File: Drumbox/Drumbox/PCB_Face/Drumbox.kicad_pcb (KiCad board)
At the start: 2 copper layers, 199.4 x 123.2 mm, 103 parts, among them J1 Bass IN, J10 HiHat IN, J12 Conn_01x08_Male, J15 Bass OUT, J16 HBonga OUT, J17 Snare OUT, J18 LBonga OUT, J19 Clave OUT, J2 HBonga IN, J20 HiHat OUT, J21 Conn_01x06_Male, J23 Conn_01x06_Male, J24 Conn_01x06_Male, J29 Conn_01x12_Male, J3 Snare IN, J31 Conn_01x08_Male, J32 Conn_01x06_Male, J4 Aux-IN, J5 FilterCV, J6 Conn_01x12_Male, J7 Mono-Out, J8 LBonga IN, J9 Clave IN, Q10 2N3904, Q11 2N3904, Q12 2N3904, Q7 2N3904, Q8 2N3904, Q9 2N3904, SW1 Mute-1, SW10 Fx2, SW11 Fx4, SW12 Fx6, SW13 Hpass/Lpass Switch, SW14 Stupid ON/OFF, SW15 Echo ON/OFF, SW2 Mute-2, SW3 Mute-3, SW4 Mute-4, SW5 Mute-5, SW6 Mute-6, SW7 Fx1, SW8 Fx3, SW9 Fx5

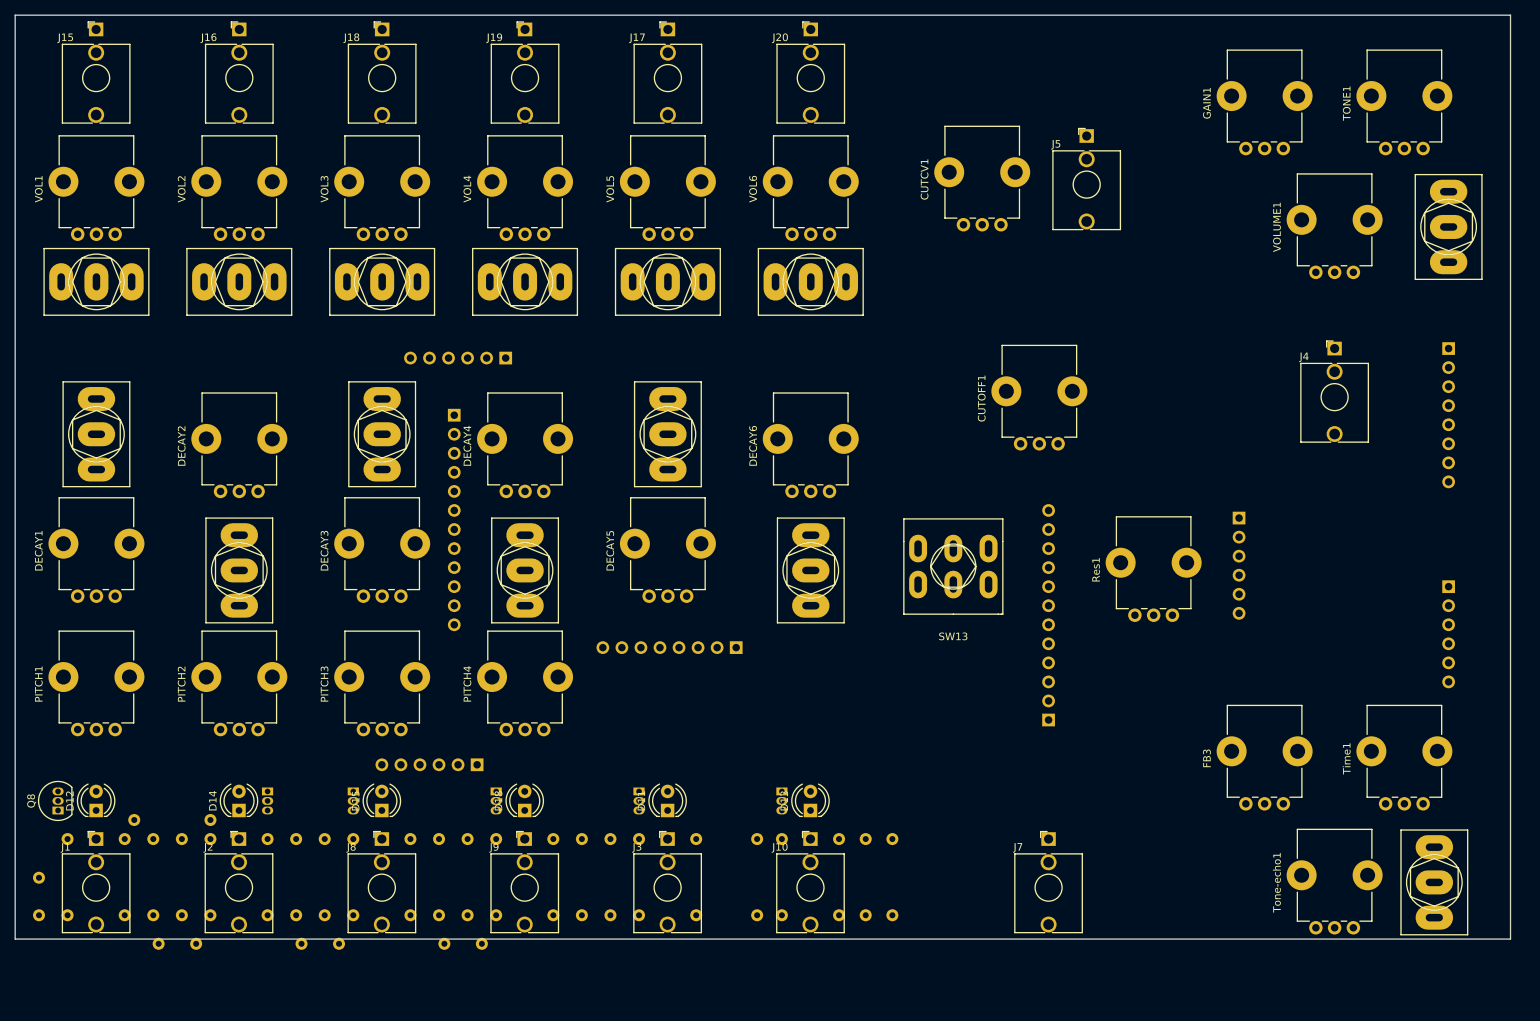
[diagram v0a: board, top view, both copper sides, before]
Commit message: big change before restart in individual modules
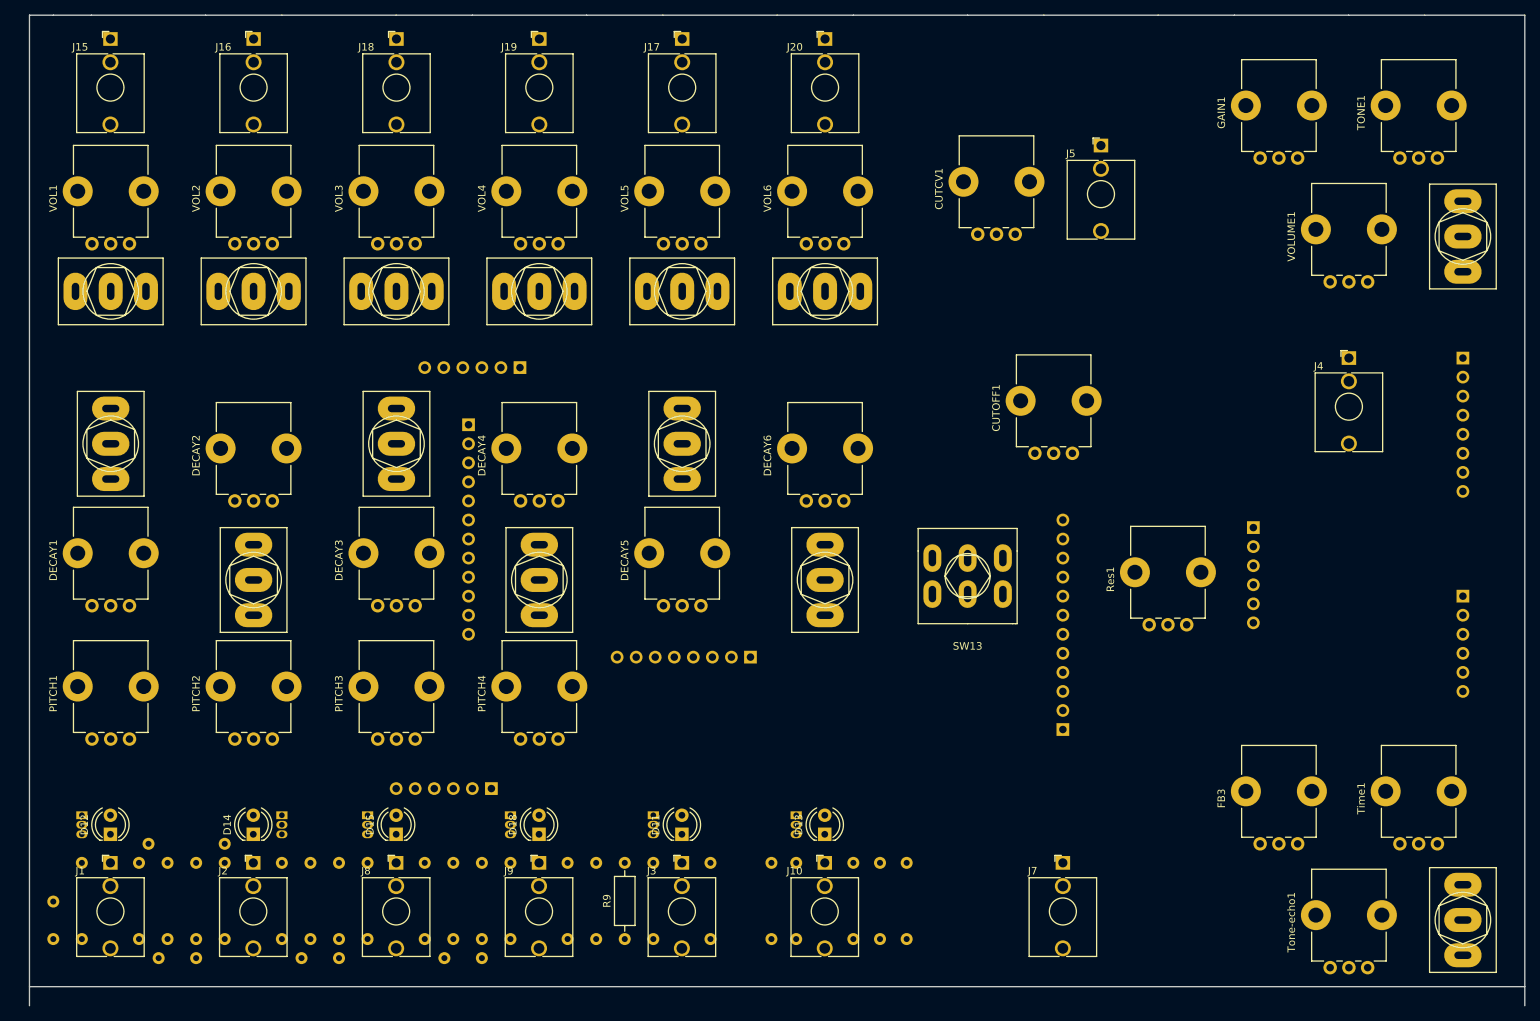
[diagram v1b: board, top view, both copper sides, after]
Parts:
- Q8: moved to B.Cu
- R9: moved to F.Cu
- moved SW15 6.30 mm to (228.6, 151.1)
- moved FB3 5.66 mm to (206.6, 141.0)
- moved Time1 5.66 mm to (225.2, 141.0)
- moved Tone-echo1 5.65 mm to (215.9, 157.5)
- moved J24 3.70 mm to (99.1, 133.6)
- moved R11 3.70 mm to (63.5, 141.0)
- moved R59 3.70 mm to (128.3, 153.7)
- moved C1 3.70 mm to (40.6, 153.7)
- moved D12 3.70 mm to (48.3, 139.7)
- moved D13 3.70 mm to (143.5, 139.7)
- moved D14 3.70 mm to (67.3, 139.7)
- moved D15 3.70 mm to (86.4, 139.7)
- moved D18 3.70 mm to (105.4, 139.7)
- moved J1 3.70 mm to (48.3, 143.5)
- moved J10 3.70 mm to (143.5, 143.5)
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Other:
- board size 199.4 x 123.2 mm -> 199.4 x 132.1 mm
